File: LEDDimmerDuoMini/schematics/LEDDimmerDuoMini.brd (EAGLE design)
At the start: 82.2 x 22.9 mm, 13 parts, among them IC1 7805T, T1 2N3904, T2 2N3904

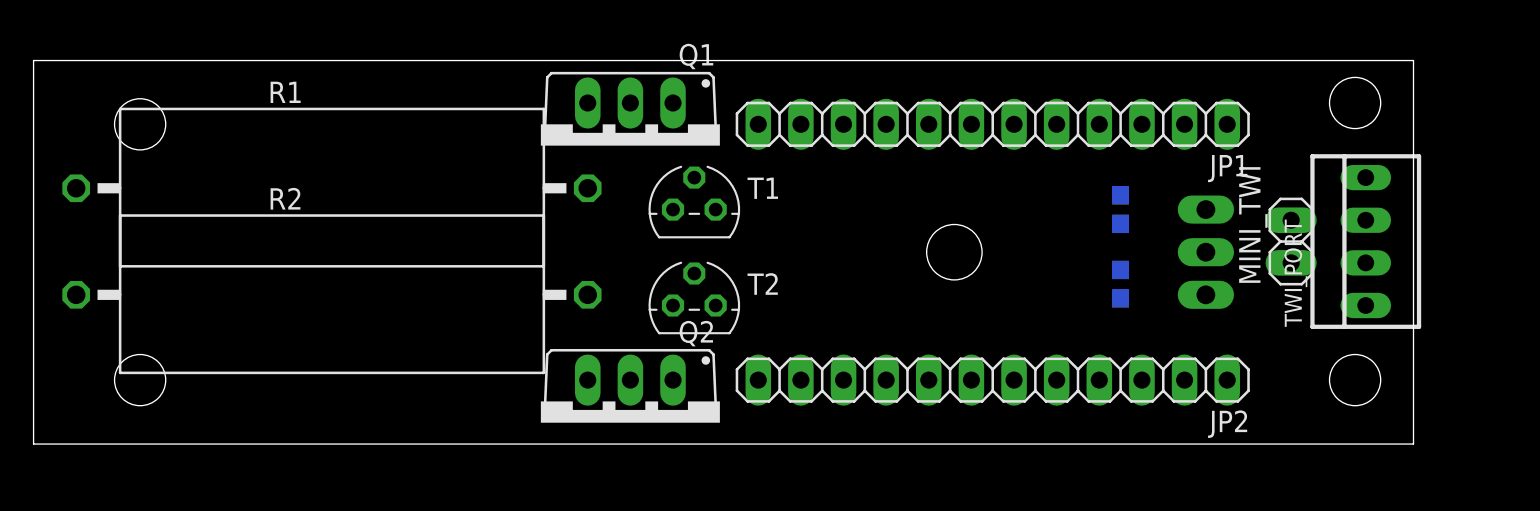
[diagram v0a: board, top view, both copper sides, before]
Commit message: Update before LED flaate testen
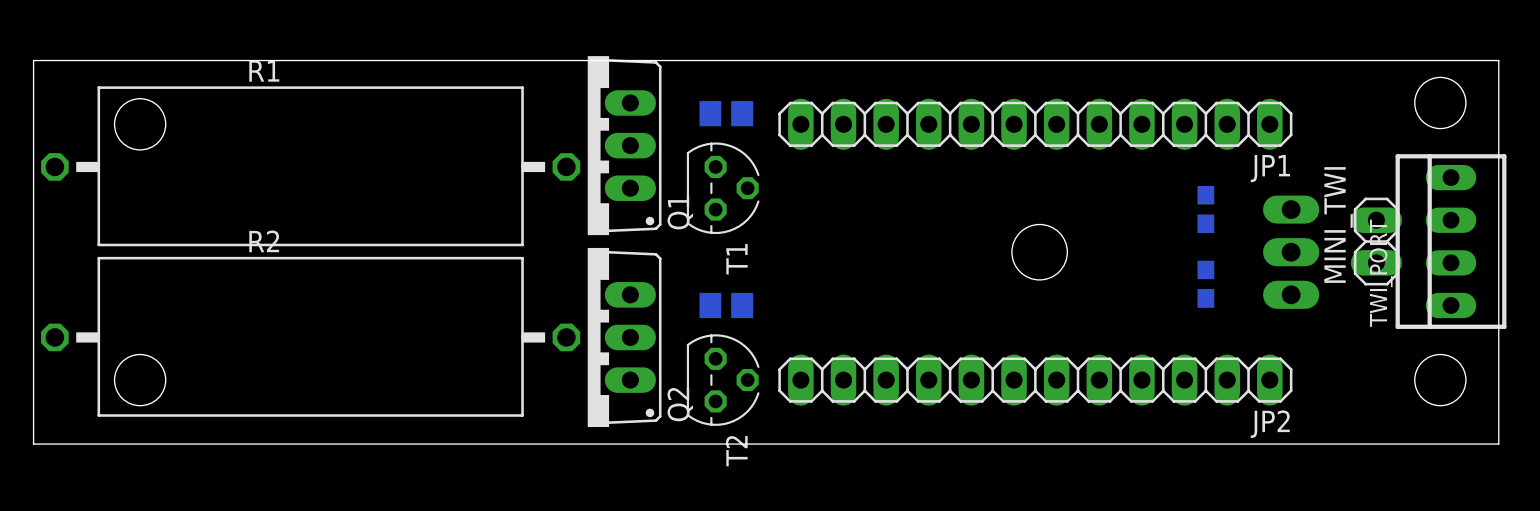
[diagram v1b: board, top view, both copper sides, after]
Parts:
- added R3, R4: (no value), eagle-ltspice:R0805
- moved Q2 5.68 mm to (33.0, 6.35), turned to 90 degrees
- moved C2 5.08 mm to (69.8, 14.0)
- moved C3 5.08 mm to (69.8, 9.53)
- moved IC1 5.08 mm to (64.8, 11.4)
- moved MINI_TWI 5.08 mm to (80.0, 12.1)
- moved TWI_PORT 5.08 mm to (84.5, 12.1)
- moved T2 4.62 mm to (40.6, 3.81), turned to 270 degrees
- moved R2 2.84 mm to (16.5, 6.35)
- moved JP1 2.54 mm to (59.7, 19.1)
- moved JP2 2.54 mm to (59.7, 3.81)
- moved Q1 2.54 mm to (33.0, 17.8), turned to 90 degrees
- moved T1 1.80 mm to (40.6, 15.2), turned to 270 degrees
- moved R1 1.80 mm to (16.5, 16.5)
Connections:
- new net N$7: Q2.G, R4.2, T2.3
- net PWM1: now also R3.1, R3.2
- net PWM2: now also R4.1; no longer Q2.G, T2.3
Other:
- board size 82.2 x 22.9 mm -> 87.3 x 22.9 mm
